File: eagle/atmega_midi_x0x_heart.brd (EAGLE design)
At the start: 100 x 80 mm, 48 parts, among them J11_VCF_CUTOFF 22-23-2021, U1 ATMEGA328P_PDIP, U2 TLV2372IP, U3 DS1267S-010+DIP14

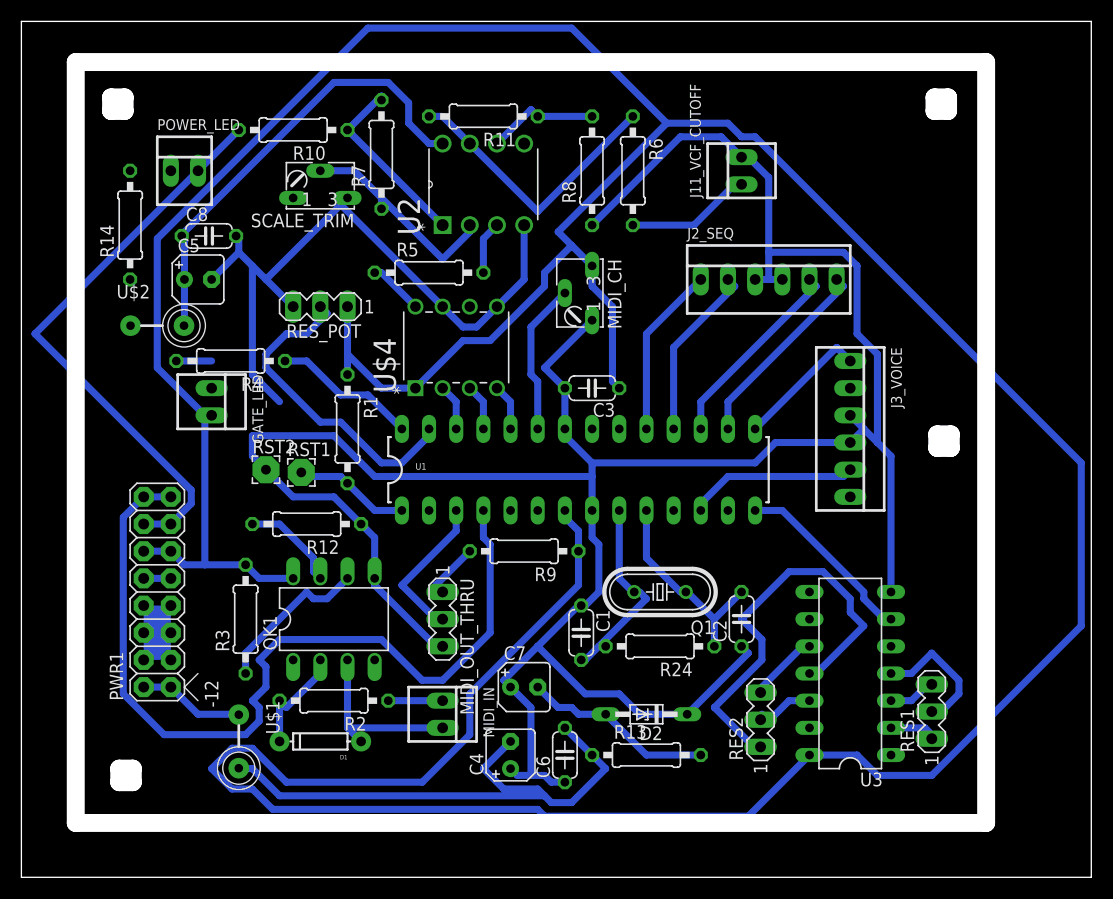
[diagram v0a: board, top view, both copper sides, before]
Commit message: high 80s autoroute
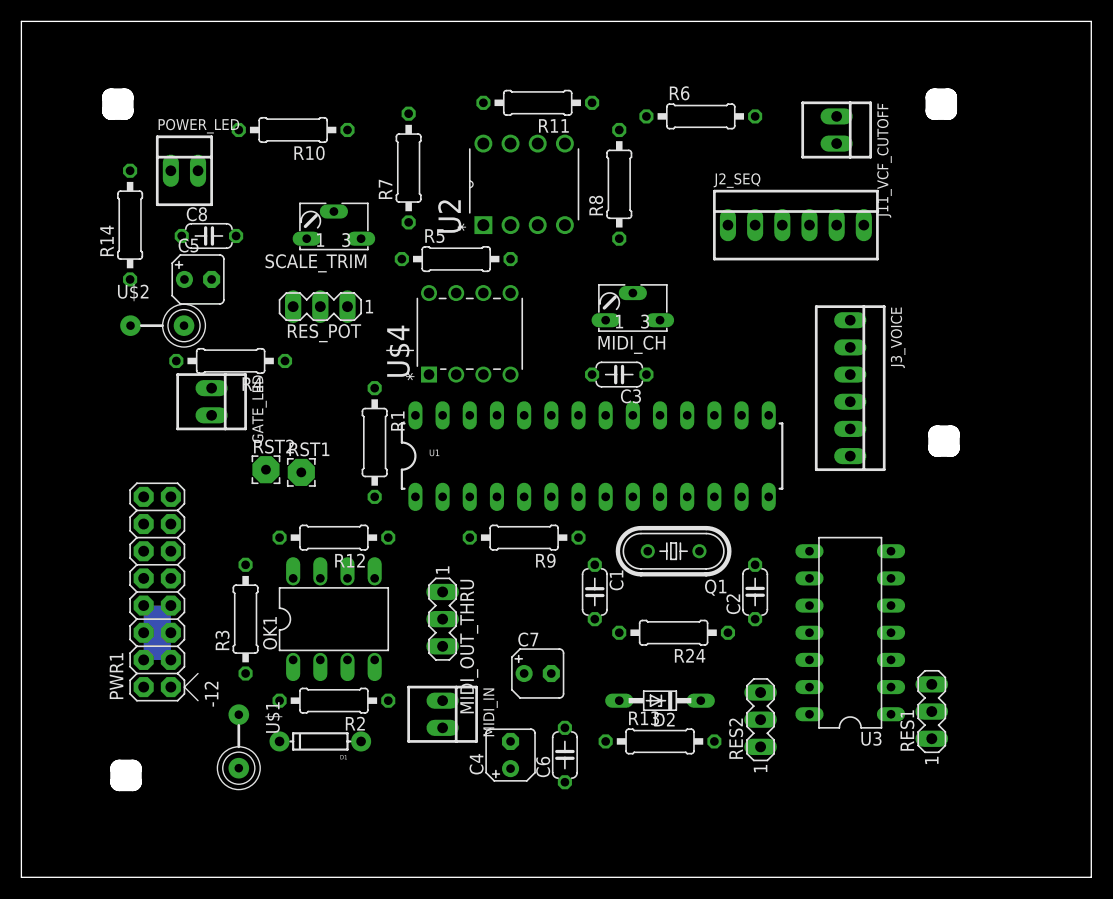
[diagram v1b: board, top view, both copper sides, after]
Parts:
- moved J11_VCF_CUTOFF 9.67 mm to (76.2, 69.8), turned to 270 degrees
- moved R6 8.13 mm to (63.5, 71.1), turned to 0 degrees
- moved J2_SEQ 5.68 mm to (72.4, 61.0)
- moved R11 5.24 mm to (48.3, 72.4)
- moved MIDI_CH 4.58 mm to (57.1, 52.1), turned to 180 degrees
- moved C1 4.02 mm to (53.6, 26.7)
- moved SCALE_TRIM 4.02 mm to (29.2, 59.7)
- moved Q1 4.02 mm to (61.0, 30.5)
- moved J3_VOICE 3.81 mm to (77.5, 45.7)
- moved U3 3.81 mm to (77.5, 22.9)
- moved U2 3.81 mm to (50.8, 68.6)
- moved R8 2.84 mm to (55.9, 64.8)
- moved C2 2.84 mm to (68.6, 26.7)
- moved C3 2.84 mm to (55.9, 47.0)
- moved R1 2.84 mm to (33.0, 40.6)
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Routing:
- net +5V: track 386.0 -> 0.00 mm
- net GND: track 316.0 -> 0.00 mm
- net N$40: track 80.8 -> 0.00 mm
- net N$15: track 54.1 -> 0.00 mm
- net -12V: track 52.7 -> 0.00 mm
- net +12V: track 42.3 -> 0.00 mm
- net N$35: track 39.8 -> 0.00 mm
- net N$38: track 30.1 -> 0.00 mm
- net N$17: track 26.4 -> 0.00 mm
- net N$12: track 20.1 -> 0.00 mm
- net N$5: track 19.3 -> 0.00 mm
- net N$4: track 18.8 -> 0.00 mm
- net N$21: track 18.7 -> 0.00 mm
- net N$23: track 18.7 -> 0.00 mm
- net N$49: track 17.9 -> 0.00 mm
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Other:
- outline, holes or cut-outs redrawn
